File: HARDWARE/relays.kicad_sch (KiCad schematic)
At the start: 60 parts, among them J15 Bulb1, J16 Bulb3, J17 Bulb3, J18 Bulb4, J19 Bulb5, J20 Bulb6, J21 Bulb7, J22 Bulb8, J23 Bulb9, J24 Bulb10, K1 SANYOU_SRD_Form_A, K10 SANYOU_SRD_Form_A, K2 SANYOU_SRD_Form_A, K3 SANYOU_SRD_Form_A, K4 SANYOU_SRD_Form_A, K5 SANYOU_SRD_Form_A, K6 SANYOU_SRD_Form_A, K7 SANYOU_SRD_Form_A, K8 SANYOU_SRD_Form_A, K9 SANYOU_SRD_Form_A, Q1 2N3904, Q10 2N3904, Q2 2N3904, Q3 2N3904, Q4 2N3904, Q5 2N3904, Q6 2N3904, Q7 2N3904, Q8 2N3904, Q9 2N3904

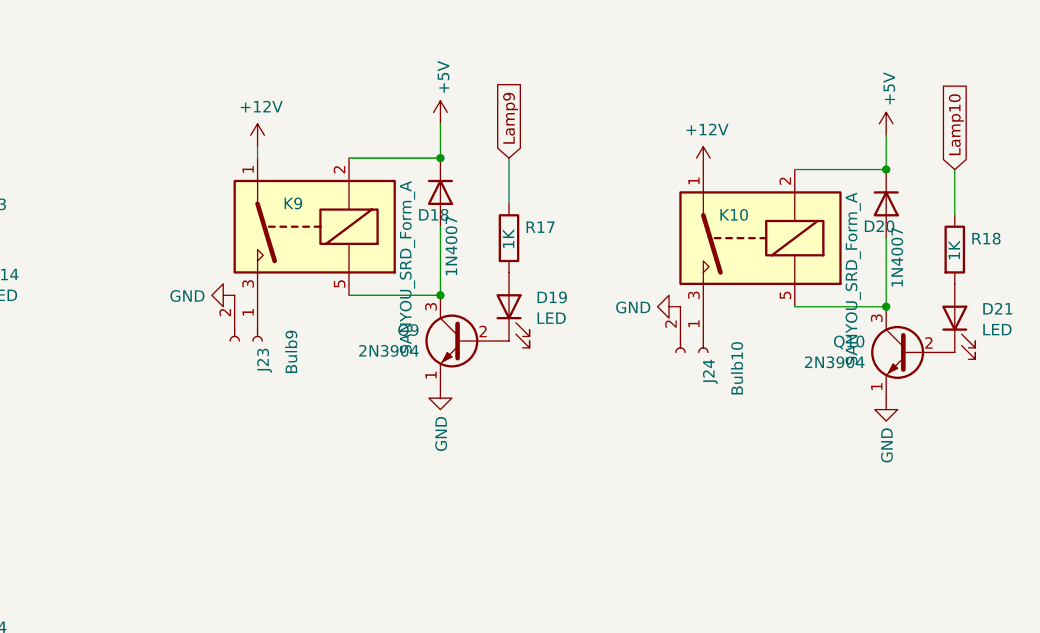
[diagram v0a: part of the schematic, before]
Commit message: Code sanitisation part 1
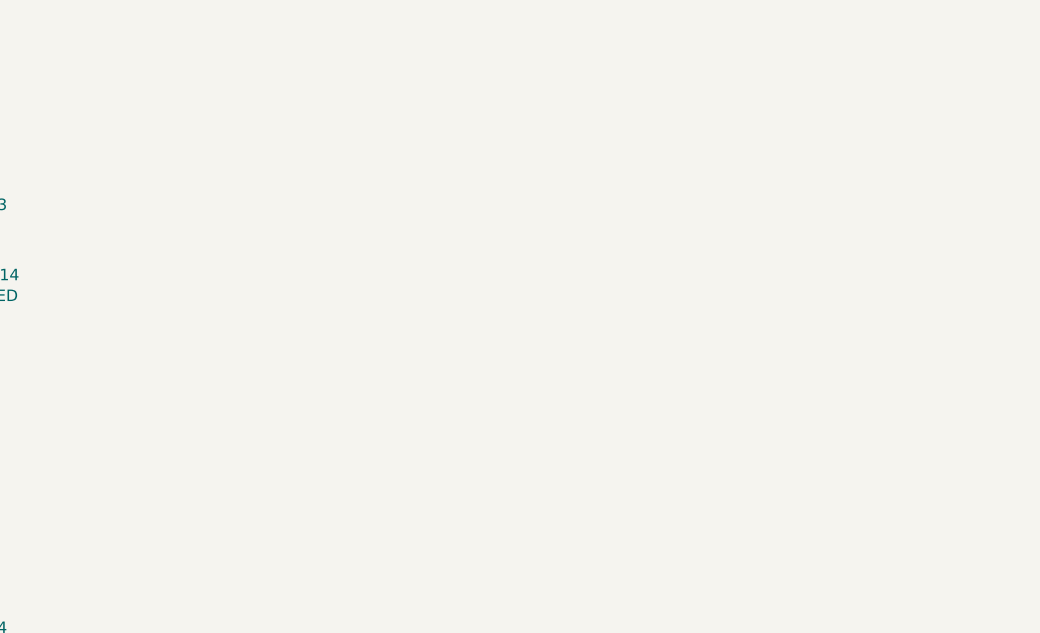
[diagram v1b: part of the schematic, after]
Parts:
- removed D18, D20: 1N4007, Diode_THT:D_DO-41_SOD81_P10.16mm_Horizontal, symbol Diode:1N4007
- removed D19, D21: LED, LED_THT:LED_D5.0mm, symbol Device:LED
- removed J23: Bulb9, Connector_Molex:Molex_KK-254_AE-6410-02A_1x02_P2.54mm_Vertical, symbol quizbuzzer-rescue:Conn_01x02_Female-Connector
- removed J24: Bulb10, Connector_Molex:Molex_KK-254_AE-6410-02A_1x02_P2.54mm_Vertical, symbol quizbuzzer-rescue:Conn_01x02_Female-Connector
- removed K10, K9: SANYOU_SRD_Form_A, Relay_THT:Relay_SPST_SANYOU_SRD_Series_Form_A, symbol Relay:SANYOU_SRD_Form_A
- removed Q10, Q9: 2N3904, Package_TO_SOT_THT:TO-92_Inline_Wide, symbol Transistor_BJT:2N3904
- removed R17, R18: 1K, Resistor_THT:R_Axial_DIN0207_L6.3mm_D2.5mm_P10.16mm_Horizontal, symbol Device:R
